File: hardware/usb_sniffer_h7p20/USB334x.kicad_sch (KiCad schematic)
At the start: 20 parts, among them J2 USB_C_Receptacle_USB2.0_16P, J3 USB_A, U2 LM2903A-VR, U3 LM2903A-VR, U4 LM2903A-VR, U5 USB3343

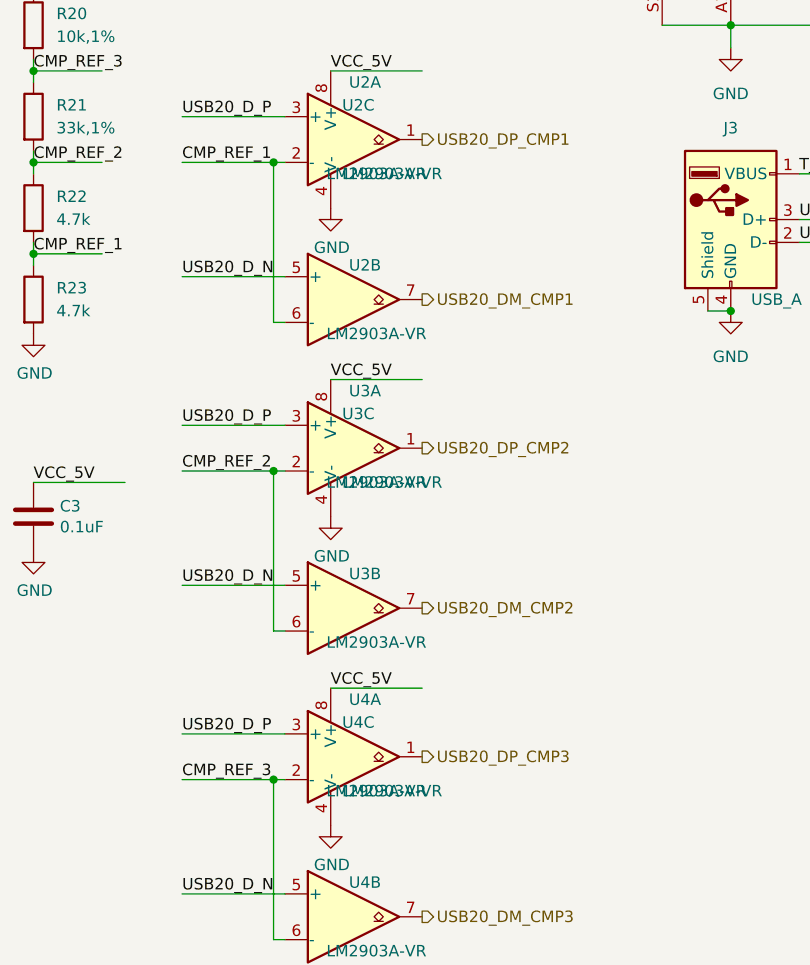
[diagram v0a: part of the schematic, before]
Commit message: [usb_sniffer_h7p20] production_files.2025620
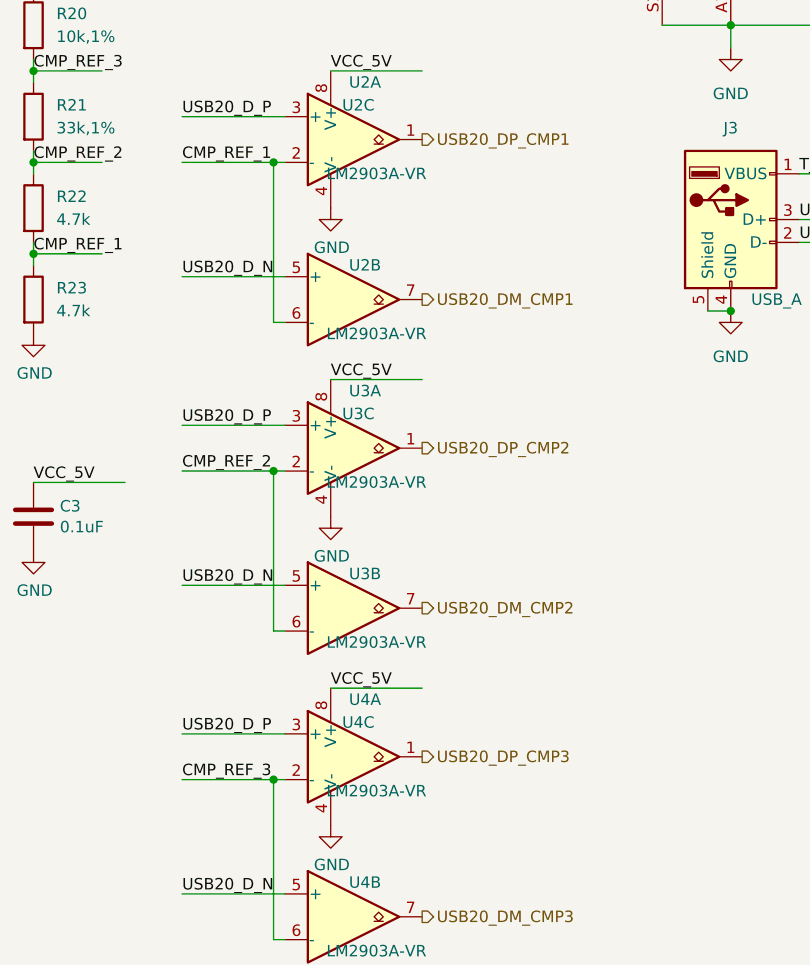
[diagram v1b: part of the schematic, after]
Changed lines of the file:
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@@
     )
     (property "Value" "LM2903A-VR" (at 58.42 142.24 0)
-      (effects (font (size 1.27 1.27)) (justify left))
+      (effects (font (size 1.27 1.27)) (justify left) hide)
     )
     (property "Footprint" "Package_SO:MSOP-8_3x3mm_P0.65mm" (at 59.69 138.43 0)
@@
     )
     (property "Value" "LM2903A-VR" (at 58.42 107.95 0)
-      (effects (font (size 1.27 1.27)) (justify left))
+      (effects (font (size 1.27 1.27)) (justify left) hide)
     )
     (property "Footprint" "Package_SO:MSOP-8_3x3mm_P0.65mm" (at 59.69 104.14 0)
@@
     )
     (property "Value" "LM2903A-VR" (at 58.42 176.53 0)
-      (effects (font (size 1.27 1.27)) (justify left))
+      (effects (font (size 1.27 1.27)) (justify left) hide)
     )
     (property "Footprint" "Package_SO:MSOP-8_3x3mm_P0.65mm" (at 59.69 172.72 0)
